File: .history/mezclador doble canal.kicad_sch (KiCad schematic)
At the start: 15 parts, among them J1 Conn_Coaxial, J2 Conn_Coaxial, J3 Conn_Coaxial, U1 NE5532

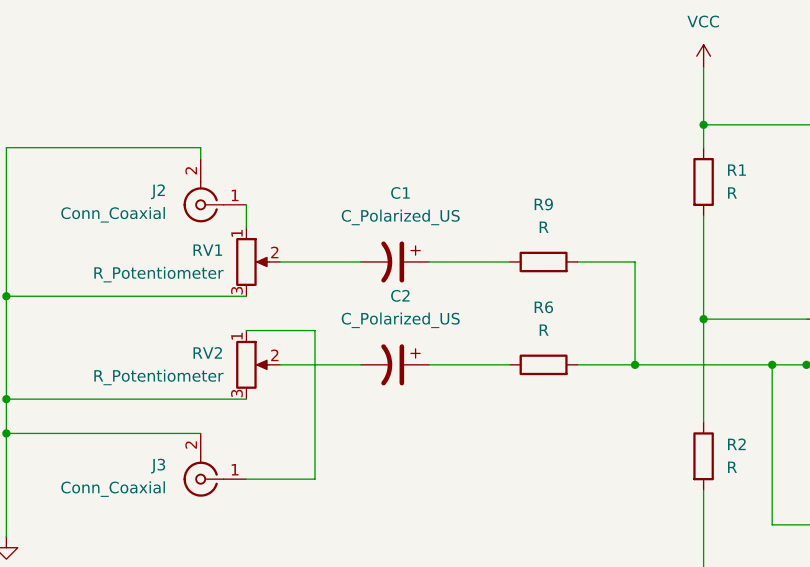
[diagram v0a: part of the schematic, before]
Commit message: completè el canal L
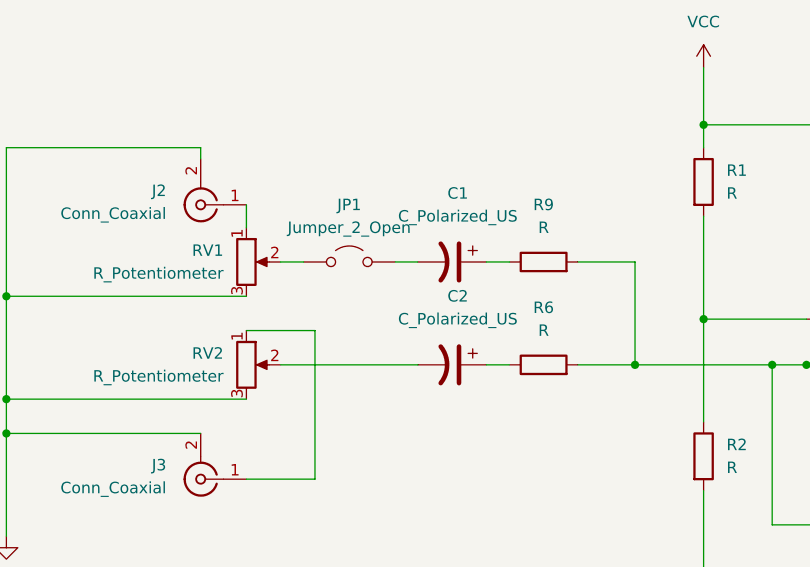
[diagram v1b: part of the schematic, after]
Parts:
- added JP1: Jumper_2_Open, personal:Jumper_Wire_10mm, symbol Jumper:Jumper_2_Open
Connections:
- net at C1.2: now also JP1.2 (B); no longer RV1.2
- new net: JP1.1 (A), RV1.2
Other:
- moved on the sheet: C1, C2
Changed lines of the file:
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@@
+	(wire
+		(pts
+			(xy 116.84 71.12) (xy 119.38 71.12)
+		)
+		(stroke
+			(width 0)
+			(type default)
+		)
+	)
 	(wire
 		(pts
@@
 	(wire
 		(pts
-			(xy 116.84 82.55) (xy 125.73 82.55)
+			(xy 116.84 82.55) (xy 132.08 82.55)
 		)
 		(stroke
@@
 	(wire
 		(pts
-			(xy 133.35 82.55) (xy 142.24 82.55)
+			(xy 139.7 82.55) (xy 142.24 82.55)
 		)
 		(stroke
@@
 	(wire
 		(pts
-			(xy 116.84 71.12) (xy 125.73 71.12)
-		)
-		(stroke
-			(width 0)
-			(type default)
-		)
-	)
-	(wire
-		(pts
 			(xy 86.36 86.36) (xy 86.36 90.17)
 		)
@@
 	(wire
 		(pts
-			(xy 133.35 71.12) (xy 142.24 71.12)
+			(xy 129.54 71.12) (xy 132.08 71.12)
+		)
+		(stroke
+			(width 0)
+			(type default)
+		)
+	)
+	(wire
+		(pts
+			(xy 139.7 71.12) (xy 142.24 71.12)
 		)
 		(stroke
@@
 	(symbol
 		(lib_id "Device:C_Polarized_US")
-		(at 129.54 71.12 270)
+		(at 135.89 71.12 270)
 		(unit 1)
 		(body_style 1)
@@
 		(fields_autoplaced yes)
 		(property "Reference" "C1"
-			(at 130.175 63.5 90)
+			(at 136.525 63.5 90)
 			(show_name no)
 			(do_not_autoplace no)
@@
 		)
 		(property "Value" "C_Polarized_US"
-			(at 130.175 66.04 90)
+			(at 136.525 66.04 90)
 			(show_name no)
 			(do_not_autoplace no)
@@
 		)
 		(property "Footprint" "Capacitor_THT:CP_Radial_D5.0mm_P2.50mm"
-			(at 129.54 71.12 0)
+			(at 135.89 71.12 0)
 			(hide yes)
 			(show_name no)
@@
 		)
 		(property "Datasheet" ""
-			(at 129.54 71.12 0)
+			(at 135.89 71.12 0)
 			(hide yes)
 			(show_name no)
@@
 		)
 		(property "Description" "Polarized capacitor, US symbol"
-			(at 129.54 71.12 0)
+			(at 135.89 71.12 0)
 			(hide yes)
 			(show_name no)
@@
 	)
 	(symbol
+		(lib_id "Jumper:Jumper_2_Open")
+		(at 124.46 71.12 0)
+		(unit 1)
+		(body_style 1)
+		(exclude_from_sim no)
+		(in_bom yes)
+		(on_board yes)
+		(in_pos_files yes)
+		(dnp no)
+		(fields_autoplaced yes)
+		(property "Reference" "JP1"
+			(at 124.46 64.77 0)
+			(show_name no)
+			(do_not_autoplace no)
+			(effects
+				(font
+					(size 1.27 1.27)
+				)
+			)
+		)
+		(property "Value" "Jumper_2_Open"
+			(at 124.46 67.31 0)
+			(show_name no)
+			(do_not_autoplace no)
+			(effects
+				(font
+					(size 1.27 1.27)
+				)
+			)
+		)
+		(property "Footprint" "personal:Jumper_Wire_10mm"
+			(at 124.46 71.12 0)
+			(hide yes)
+			(show_name no)
+			(do_not_autoplace no)
+			(effects
+				(font
+					(size 1.27 1.27)
+				)
+			)
+		)
+		(property "Datasheet" ""
+			(at 124.46 71.12 0)
+			(hide yes)
+			(show_name no)
+			(do_not_autoplace no)
+			(effects
+				(font
+					(size 1.27 1.27)
+				)
+			)
+		)
+		(property "Description" "Jumper, 2-pole, open"
+			(at 124.46 71.12 0)
+			(hide yes)
+			(show_name no)
+			(do_not_autoplace no)
+			(effects
+				(font
+					(size 1.27 1.27)
+				)
+			)
+		)
+		(pin "1"
+		)
+		(pin "2"
+		)
+		(instances
+			(project "mezclador doble canal"
+				(path "/1fd6db7d-bb33-43be-9c70-fde303eb7f84"
+					(reference "JP1")
+					(unit 1)
+				)
+			)
+		)
+	)
+	(symbol
 		(lib_id "power:GND")
 		(at 86.36 101.6 0)
@@
 	(symbol
 		(lib_id "Device:C_Polarized_US")
-		(at 129.54 82.55 270)
+		(at 135.89 82.55 270)
 		(unit 1)
 		(body_style 1)
@@
 		(fields_autoplaced yes)
 		(property "Reference" "C2"
-			(at 130.175 74.93 90)
+			(at 136.525 74.93 90)
 			(show_name no)
 			(do_not_autoplace no)
@@
 		)
 		(property "Value" "C_Polarized_US"
-			(at 130.175 77.47 90)
+			(at 136.525 77.47 90)
 			(show_name no)
 			(do_not_autoplace no)
@@
 		)
 		(property "Footprint" "Capacitor_THT:CP_Radial_D5.0mm_P2.50mm"
-			(at 129.54 82.55 0)
+			(at 135.89 82.55 0)
 			(hide yes)
 			(show_name no)
@@
 		)
 		(property "Datasheet" ""
-			(at 129.54 82.55 0)
+			(at 135.89 82.55 0)
 			(hide yes)
 			(show_name no)
@@
 		)
 		(property "Description" "Polarized capacitor, US symbol"
-			(at 129.54 82.55 0)
-			(hide yes)
-			(show_name no)
+			(at 135.89 82.55 0)
+			(hide yes)
+			(show_name no)
